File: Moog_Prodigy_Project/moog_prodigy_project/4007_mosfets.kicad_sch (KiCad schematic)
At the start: 24 parts, among them Q12 BC327, Q13 BC327, SW10 FINAL DECAY SWITCH, SW9 FINAL DECAY SWITCH, U18 OPA184, U19 OPA184

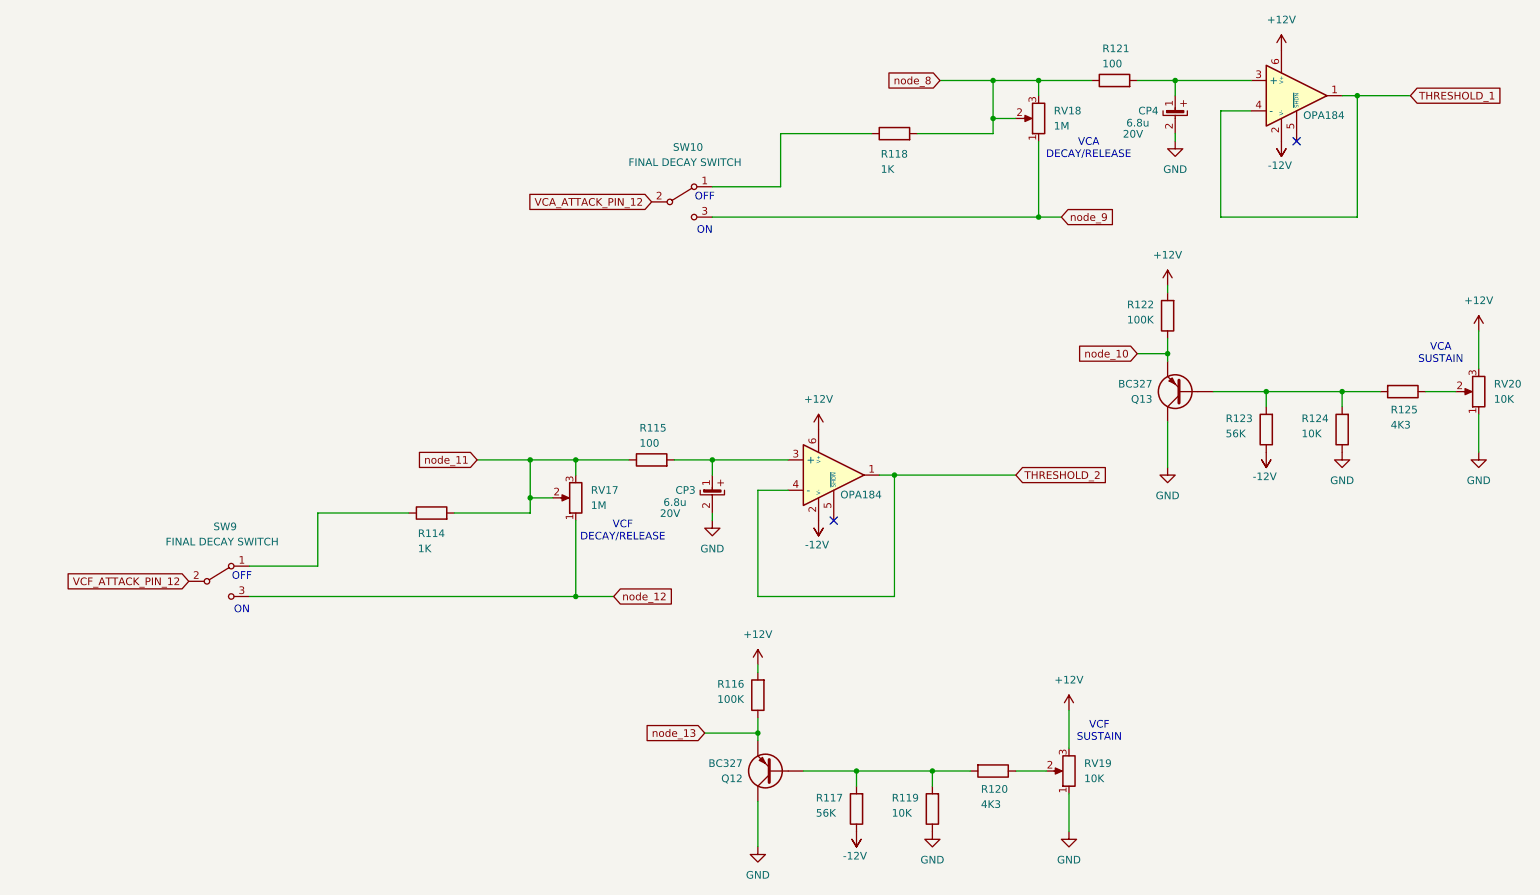
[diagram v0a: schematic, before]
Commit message: Latest checkpoints update 05.06.2026
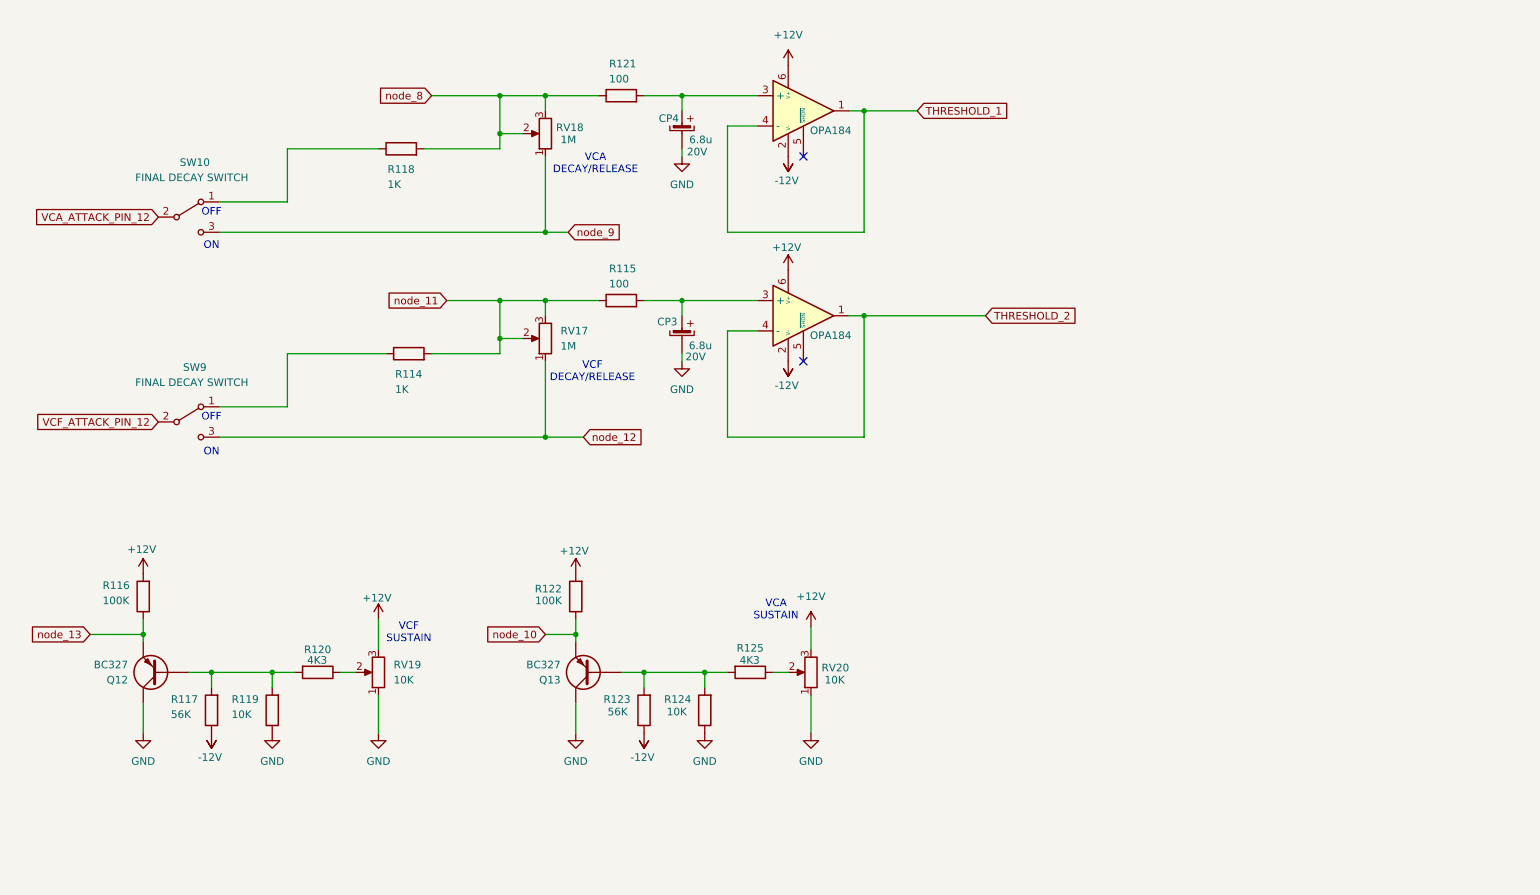
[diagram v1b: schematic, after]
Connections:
- net GND: now also CP3., CP4.; no longer CP3.2, CP4.2
- net at R115.2, U18.3 (+): now also CP3.; no longer CP3.1
- net at R121.2, U19.3 (+): now also CP4.; no longer CP4.1
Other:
- moved on the sheet: Q12, Q13, R114, R115, R116, R117, R118, R119, R120, R121, R122, R123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
